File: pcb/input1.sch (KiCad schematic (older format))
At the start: 28 parts, among them Q1 BC847, Q2 BC847, U10 SN74LVCC4245APW, U11 SN74LVCC4245APW, U14 SN74LVCC4245APW, U18 SN74LVCC4245APW, U19 SN74LVC3G17, U4 PCEngineExpansion, U9 SN74LVCC4245APW

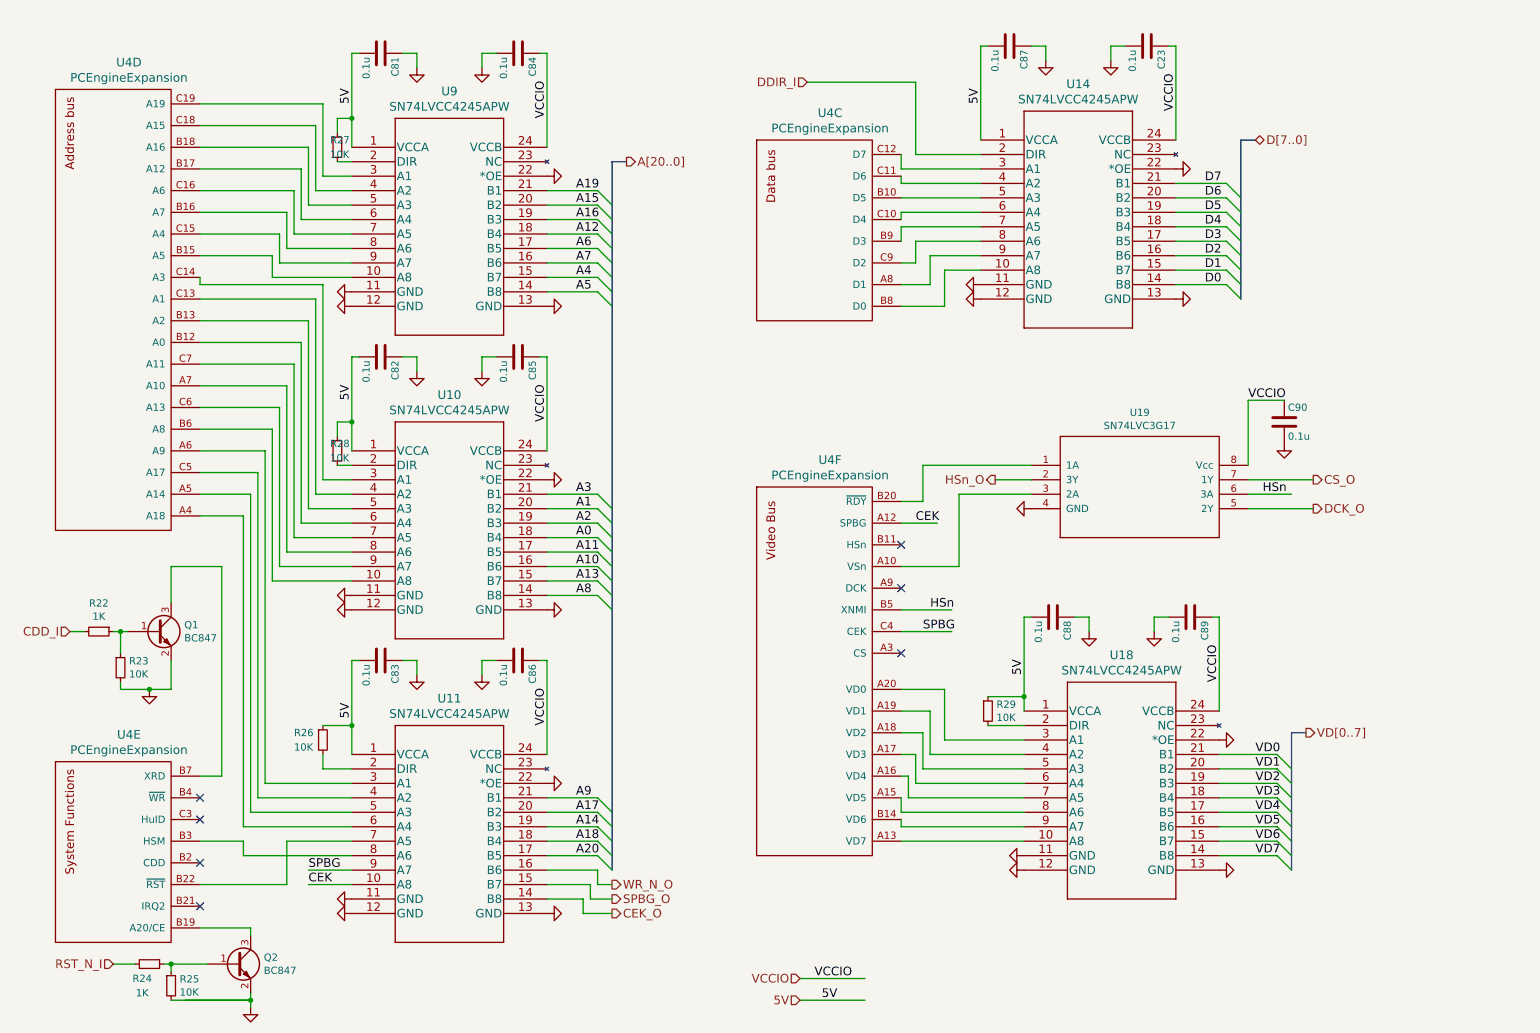
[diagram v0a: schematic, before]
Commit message: New layout
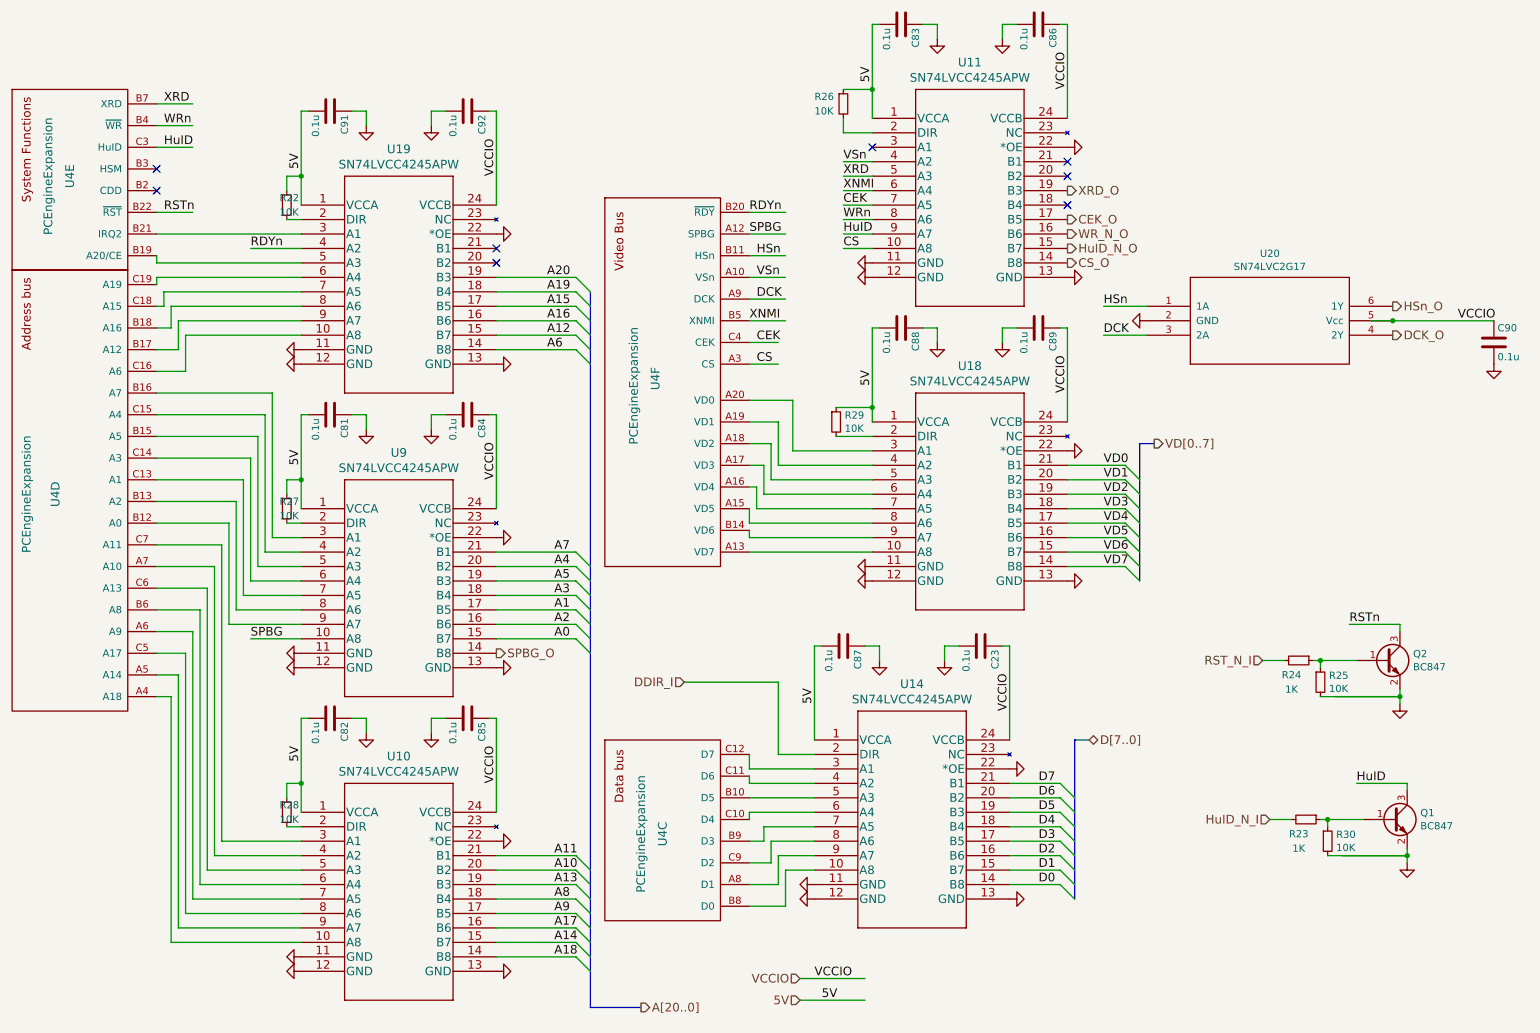
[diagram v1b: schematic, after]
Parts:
- removed U19: SN74LVC3G17, custom_components:SSOP-8_3x3mm_Pitch0.65mm, symbol custom_components:SN74LVC3G17
- added C91, C92: 0.1u, custom_components:SM0603_Capa_libcms, symbol pcehd-rescue:C-Device
- added R30: 10K, custom_components:SM0603_Resistor_libcms, symbol Device:R_Small
- added U19: SN74LVCC4245APW, custom_components:SN74LVCC4245APW, symbol custom_components:SN74LVCC4245APW
- added U20: SN74LVC2G17, custom_components:SOT-23-6_Handsoldering, symbol custom_components:SN74LVC2G17
- R22: value 1K -> 10K
- R23: value 10K -> 1K
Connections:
- net labels added: CS, DCK, HuID, HuID_N_I, HuID_N_O, RDYn, RSTn, VSn, WRn, XNMI, XRD, XRD_O
- net labels removed: CDD_I
- wire segments 250 -> 255
- no-connect marks 7 -> 8
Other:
- moved on the sheet: C23, C81, C82, C83, C84, C85, C86, C87, C88, C89, C90, Q2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
